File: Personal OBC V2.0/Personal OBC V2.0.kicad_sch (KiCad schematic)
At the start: 13 parts, among them J2 Screw_Terminal_01x06, U1 STM32F042G6Ux, U2 MS560702BA03-50, U3 AP2210N-3.3TRG1

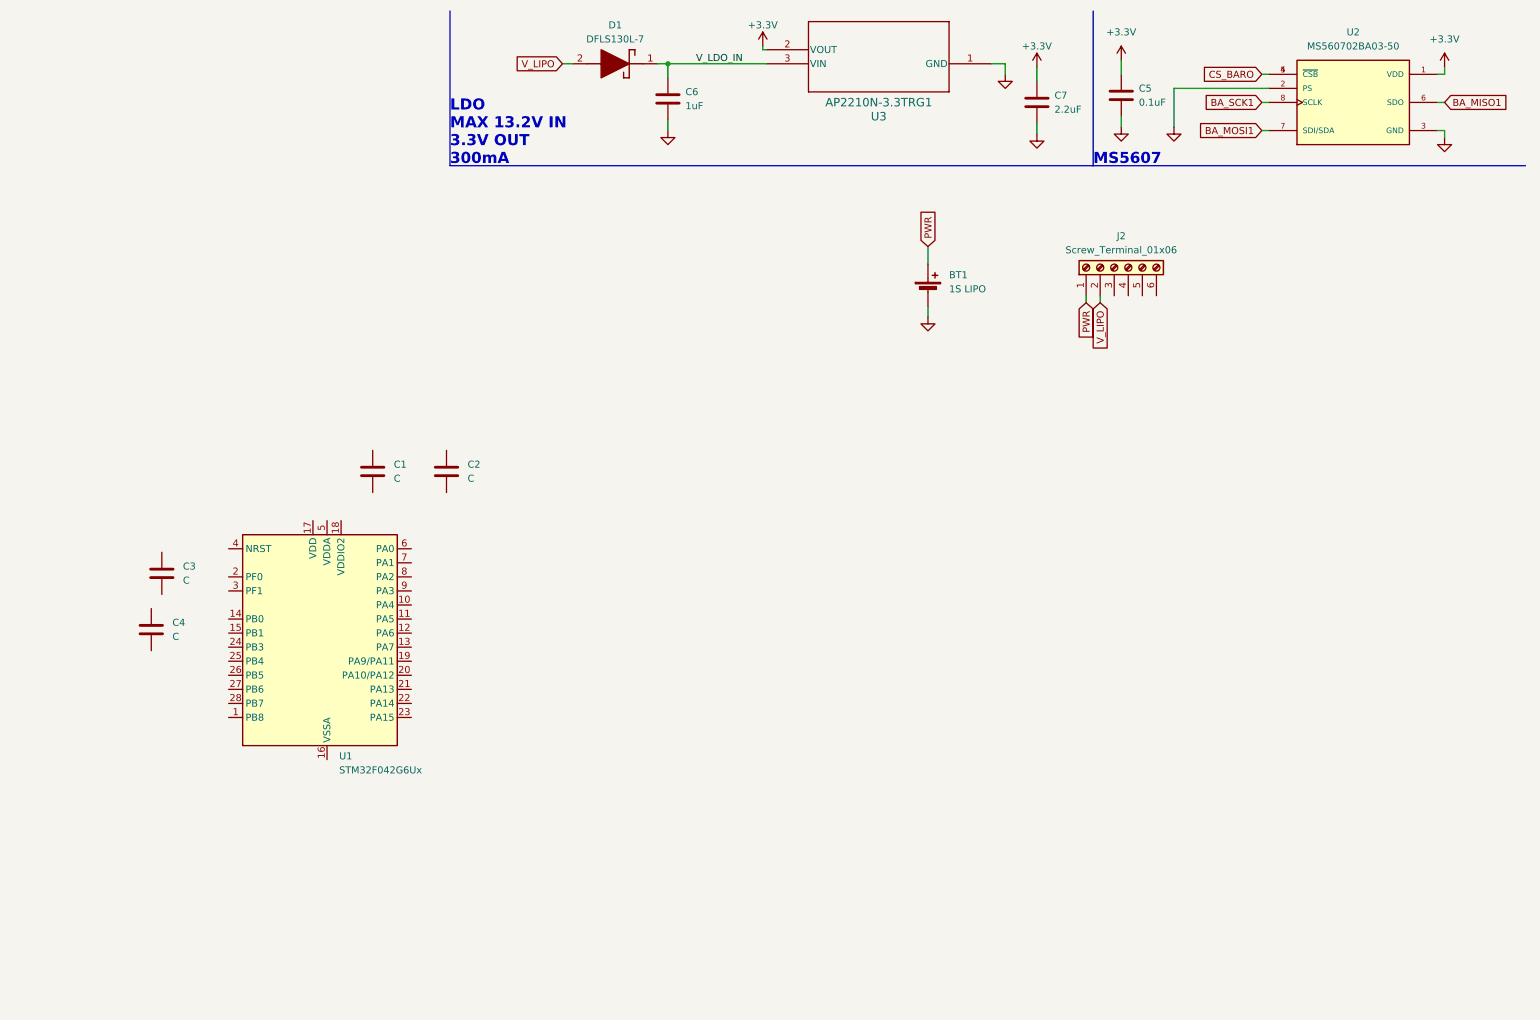
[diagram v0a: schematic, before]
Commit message: Aaaaaa
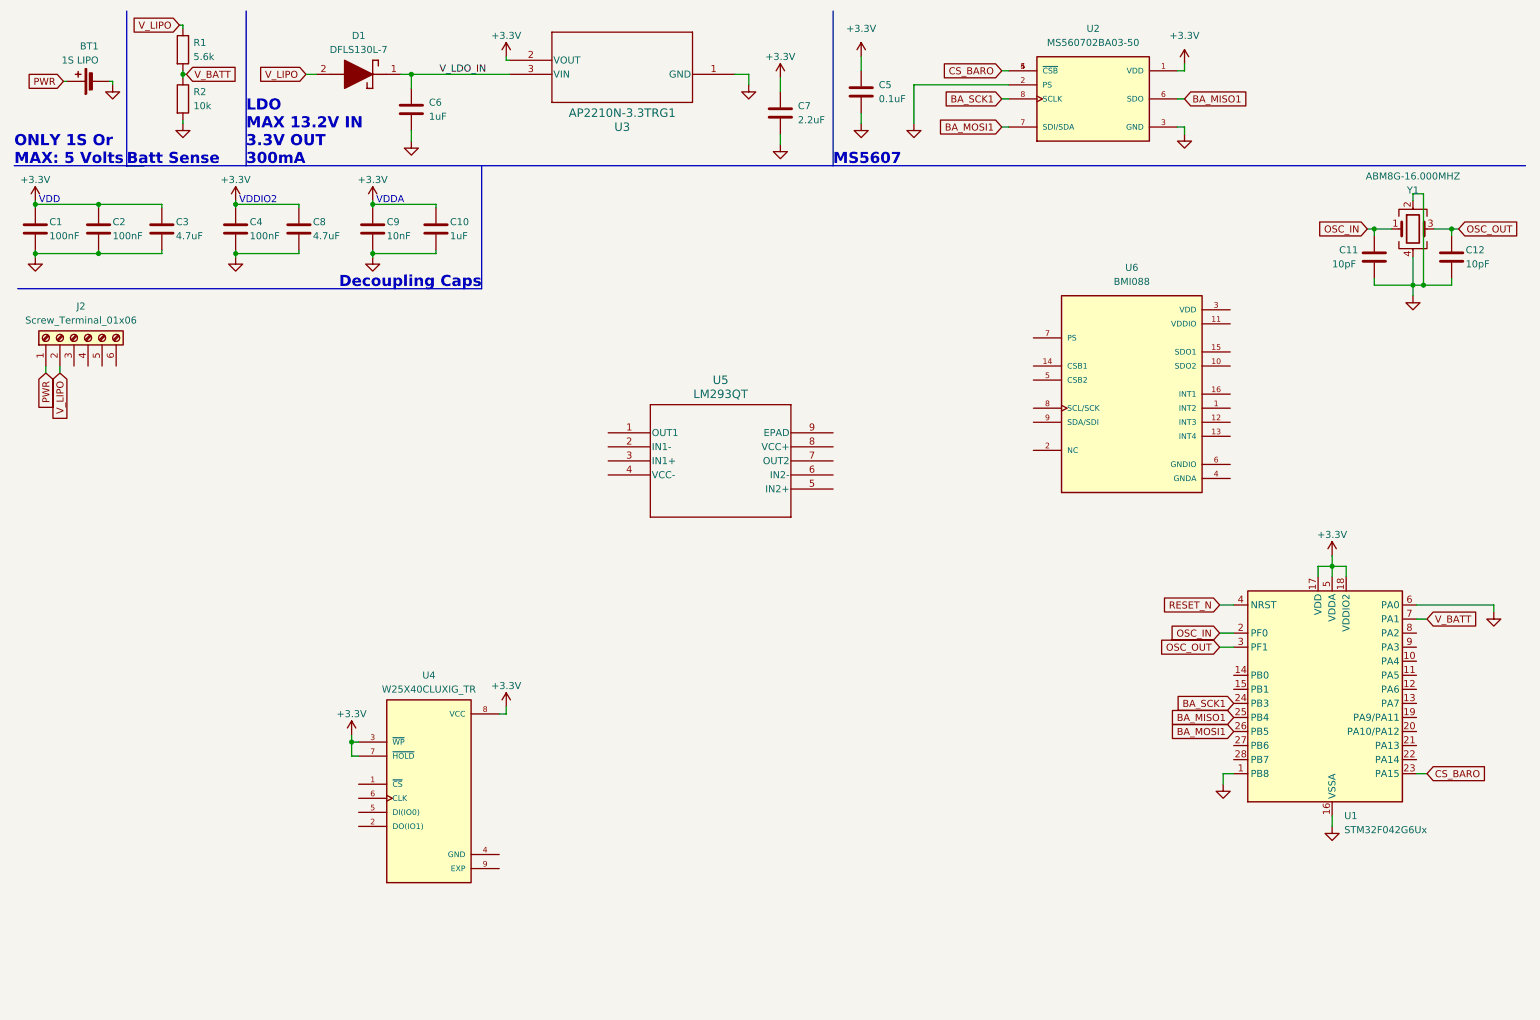
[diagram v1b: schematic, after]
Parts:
- added C10: 1uF, symbol Device:C
- added C11, C12: 10pF, symbol Device:C
- added C8: 4.7uF, symbol Device:C
- added C9: 10nF, symbol Device:C
- added R1: 5.6k, symbol Device:R
- added R2: 10k, symbol Device:R
- added U4: W25X40CLUXIG_TR, W25X40CLUXIG_TR:PSON50P300X200X60-9N, symbol W25X40CLUXIG TR:W25X40CLUXIG_TR
- added U5: LM293QT, DFN8_2P16X2P16X0P5_STM, symbol LM293QT:LM293QT
- added U6: BMI088, BMI088:PQFN50P450X300X100-16N, symbol BMI088:BMI088
- added Y1: ABM8G-16.000MHZ, Crystal:Crystal_SMD_Abracon_ABM8G-4Pin_3.2x2.5mm, symbol Device:Crystal_GND24
- C1, C2, C4: value C -> 100nF
- C3: value C -> 4.7uF
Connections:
- net +3.3V: now also C1.1, C2.1, C3.1, C4.1, U1.17 (VDD), U1.18 (VDDIO2), U1.5 (VDDA), C10.1, C8.1, C9.1, U4.3 (~{WP}), U4.7 (~{HOLD}), U4.8 (VCC)
- net BA_MISO1: now also U1.25 (PB4)
- net BA_MOSI1: now also U1.26 (PB5)
- net BA_SCK1: now also U1.24 (PB3)
- net CS_BARO: now also U1.23 (PA15)
- net GND: now also C1.2, C2.2, C3.2, C4.2, U1.1 (PB8), U1.16 (VSSA), U1.6 (PA0), C10.2, C11.2, C12.2, C8.2, C9.2, R2.2, Y1.2, Y1.4
- net V_LIPO: now also R1.1
- net OSC_IN: now reaches U1.2 (PF0)
- net OSC_IN: now also C11.1, Y1.1
- net OSC_OUT: now reaches U1.3 (PF1)
- net OSC_OUT: now also C12.1, Y1.3
- net RESET_N: now reaches U1.4 (NRST)
- net V_BATT: now reaches U1.7 (PA1)
- net V_BATT: now also R1.2, R2.1
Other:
- note added: "Batt Sense"
- note added: "Decoupling Caps"
- note added: "ONLY 1S Or MAX: 5 Volts"
- note added: "VDD"
- note added: "VDDA"
- note added: "VDDIO2"
- moved on the sheet: BT1, C1, C2, C3, C4, C5, C6, C7, D1, J2, U1, U2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

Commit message: Piss bot
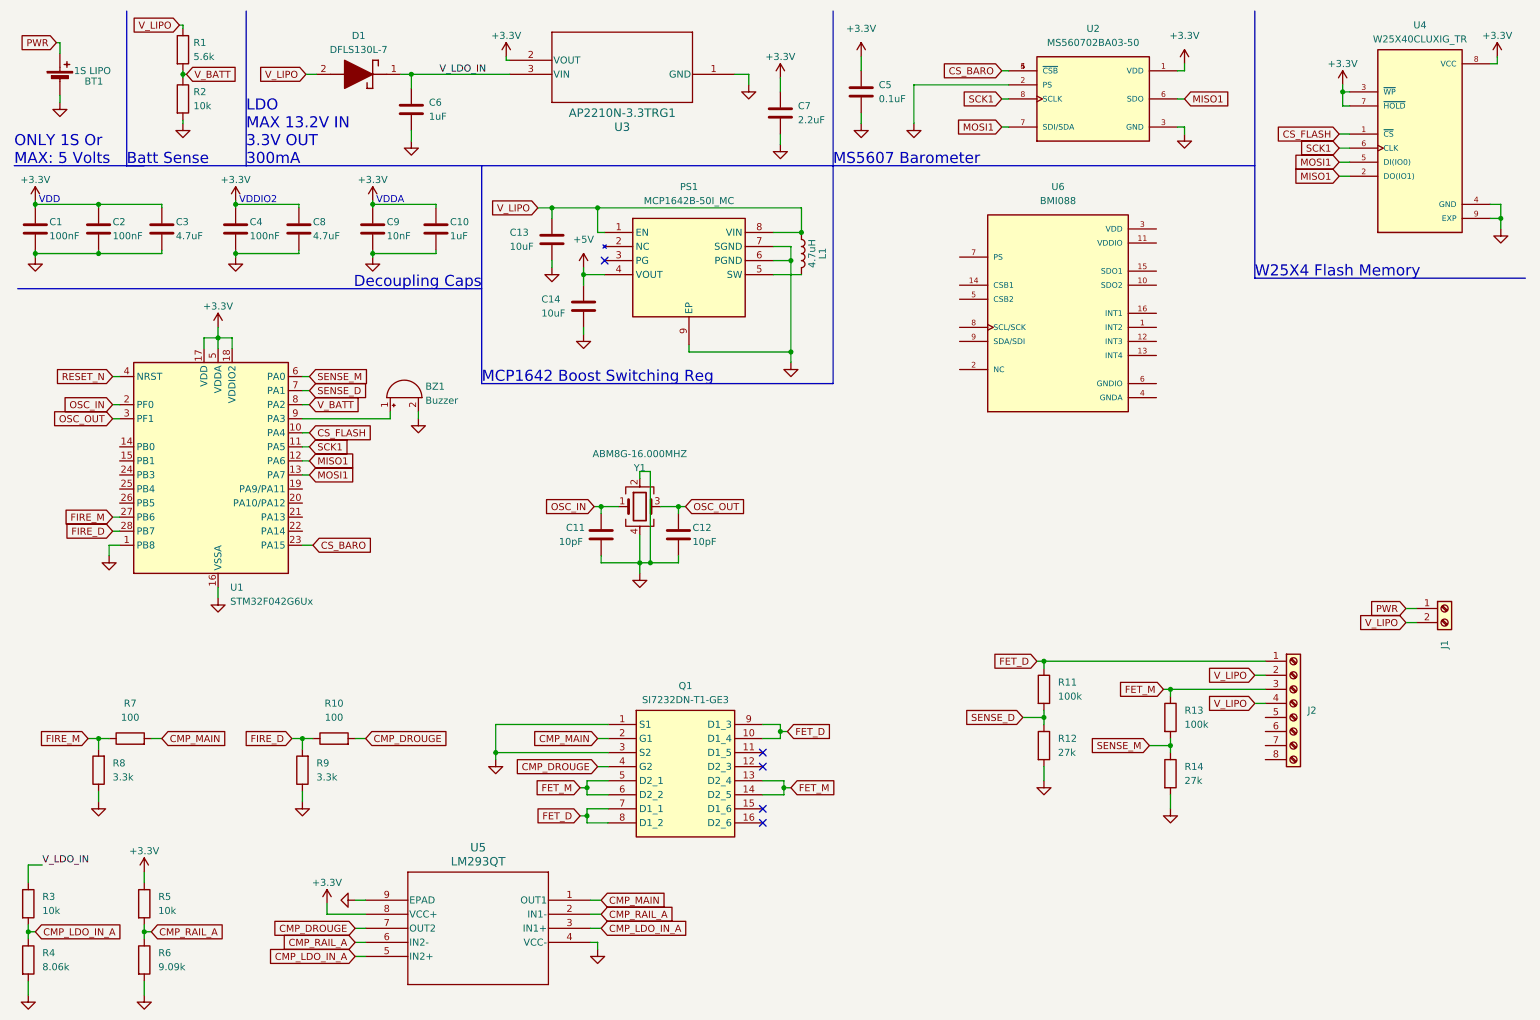
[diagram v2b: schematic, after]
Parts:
- removed J2: Screw_Terminal_01x06, symbol Connector:Screw_Terminal_01x06
- added BZ1: Buzzer, symbol Device:Buzzer
- added C13, C14: 10uF, symbol Device:C
- added J1: Screw_Terminal_01x02, symbol Connector:Screw_Terminal_01x02
- added J2: Screw_Terminal_01x04, symbol Connector:Screw_Terminal_01x08
- added L1: 4.7uH, symbol Device:L
- added PS1: MCP1642B-50I_MC, SON50P300X200X100-9N-D, symbol MCP1642B-50I_MC:MCP1642B-50I_MC
- added Q1: SI7232DN-T1-GE3, SI7232DNT1GE3, symbol SI7232DN-T1-GE3:SI7232DN-T1-GE3
- added R10, R7: 100, symbol Device:R
- added R11, R13: 100k, symbol Device:R
- added R12, R14: 27k, symbol Device:R
- added R3, R5: 10k, symbol Device:R
- added R4: 8.06k, symbol Device:R
- added R6: 9.09k, symbol Device:R
- added R8, R9: 3.3k, symbol Device:R
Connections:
- net +3.3V: now also U5.8 (VCC+), R5.1
- net GND: now also U4.4 (GND), U4.9 (EXP), U5.4 (VCC-), U5.9 (EPAD), BZ1.2 (+), C13.2, C14.2, PS1.6 (PGND), PS1.7 (SGND), PS1.9 (EP), Q1.1 (S1), Q1.3 (S2), R12.2, R14.2, R4.2, R6.2, R8.1, R9.1; no longer U1.6 (PA0)
- net PWR: now also J1.1 (Pin_1)
- net V_BATT: now also U1.8 (PA2); no longer U1.7 (PA1)
- net V_LDO_IN: now also R3.1
- net V_LIPO: now also C13.1, J1.2 (Pin_2), J2.2 (Pin_2), J2.4 (Pin_4), L1.1, PS1.1 (EN), PS1.8 (VIN)
- net CS_FLASH: now reaches U1.10 (PA4)
- net CS_FLASH: now also U4.1 (~{CS})
- net SCK1: now reaches U1.11 (PA5)
- net SCK1: now also U2.8 (SCLK), U4.6 (CLK)
- net MISO1: now reaches U1.12 (PA6)
- net MISO1: now also U2.6 (SDO), U4.2 (DO(IO1))
- net MOSI1: now reaches U1.13 (PA7)
- net MOSI1: now also U2.7 (SDI/SDA), U4.5 (DI(IO0))
- net FIRE_M: now reaches U1.27 (PB6)
- net FIRE_M: now also R7.1, R8.2
- net FIRE_D: now reaches U1.28 (PB7)
- net FIRE_D: now also R10.1, R9.2
- net at U1.9 (PA3): now also BZ1.1 (-)
- net CMP_MAIN: now reaches U5.1 (OUT1)
- net CMP_MAIN: now also Q1.2 (G1), R7.2
- net CMP_RAIL_A: now reaches U5.2 (IN1-)
- net CMP_RAIL_A: now also U5.6 (IN2-), R5.2, R6.1
- net CMP_LDO_IN_A: now reaches U5.3 (IN1+)
- net CMP_LDO_IN_A: now also U5.5 (IN2+), R3.2, R4.1
- net CMP_DROUGE: now reaches U5.7 (OUT2)
- net CMP_DROUGE: now also Q1.4 (G2), R10.2
- net BA_MISO1: no longer names the net of U1.25 (PB4)
- net BA_MISO1: no longer U2.6 (SDO)
- net BA_MOSI1: no longer names the net of U1.26 (PB5)
- net BA_MOSI1: no longer U2.7 (SDI/SDA)
- net BA_SCK1: no longer names the net of U1.24 (PB3)
- net BA_SCK1: no longer U2.8 (SCLK)
- new net: L1.2, PS1.5 (SW)
- new net +5V: C14.1, PS1.4 (VOUT)
- new net FET_D: J2.1 (Pin_1), Q1.10 (D1_4), Q1.7 (D1_1), Q1.8 (D1_2), Q1.9 (D1_3), R11.1
- new net FET_M: J2.3 (Pin_3), Q1.13 (D2_4), Q1.14 (D2_5), Q1.5 (D2_1), Q1.6 (D2_2), R13.1
- new net SENSE_D: R11.2, R12.1, U1.7 (PA1)
- new net SENSE_M: R13.2, R14.1, U1.6 (PA0)
- no-connect marks 0 -> 5
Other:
- note added: "MCP1642 Boost Switching Reg"
- note added: "MS5607 Barometer"
- note added: "W25X4 Flash Memory"
- note removed: "MS5607"
- moved on the sheet: BT1, C11, C12, U1, U4, U5, U6, Y1

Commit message: AAAA
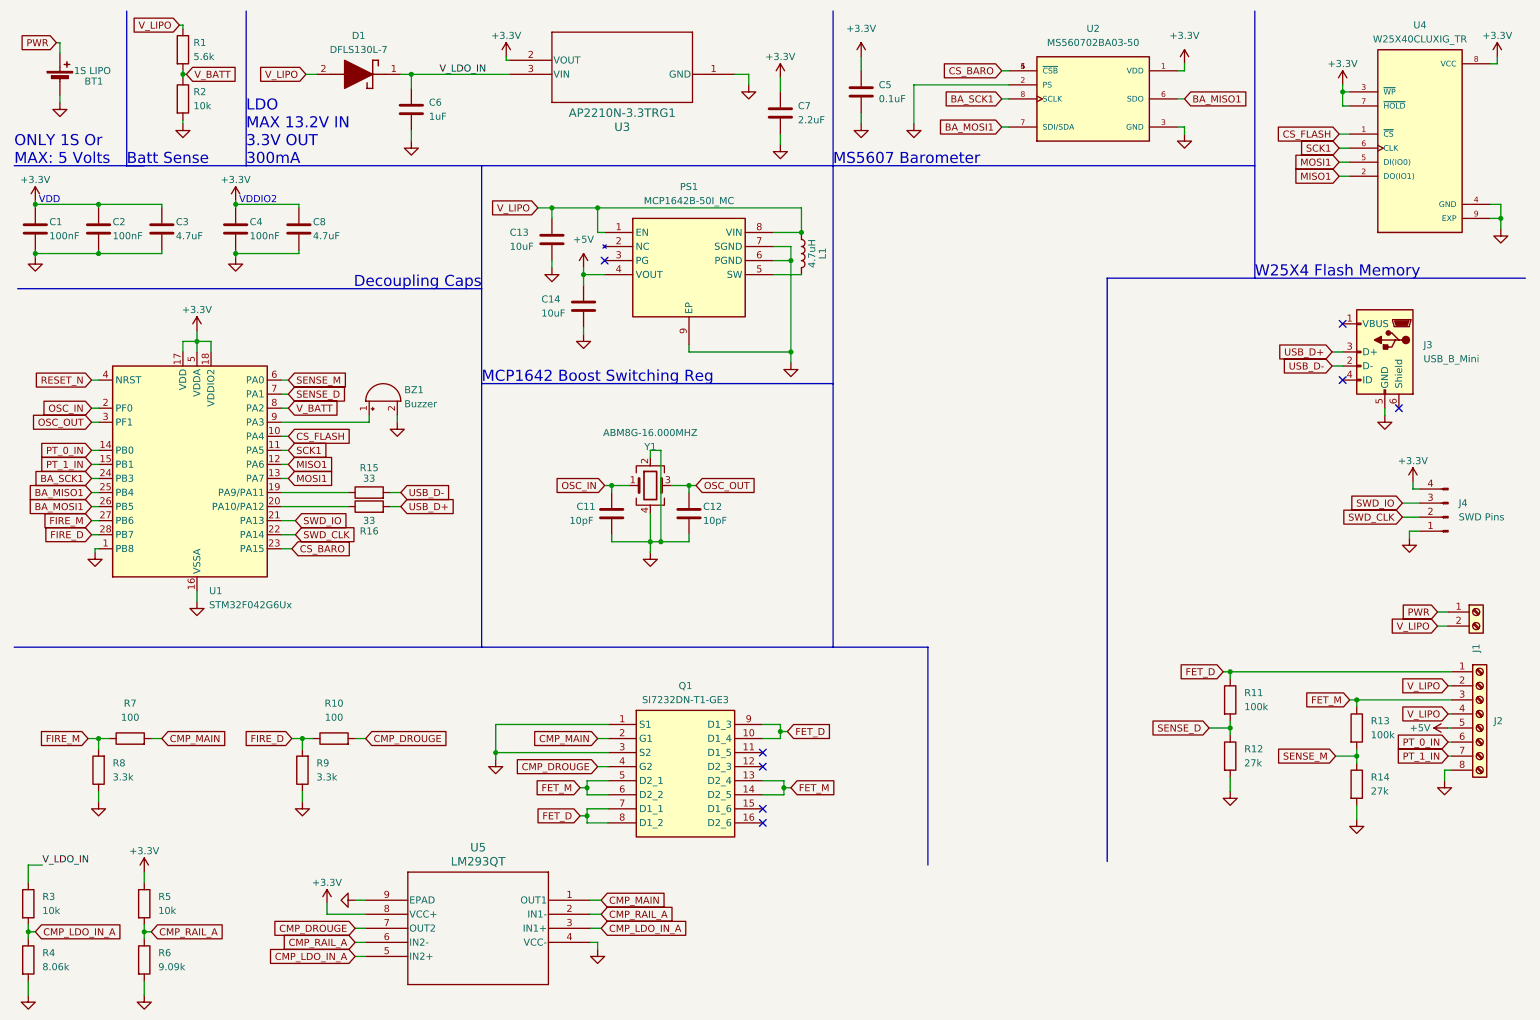
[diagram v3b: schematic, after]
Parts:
- removed C10: 1uF, symbol Device:C
- removed C9: 10nF, symbol Device:C
- removed U6: BMI088, BMI088:PQFN50P450X300X100-16N, symbol BMI088:BMI088
- added J3: USB_B_Mini, Connector_USB:USB_Micro-AB_Molex_47590-0001, symbol Connector:USB_B_Mini
- added J4: SWD Pins, symbol Connector:Conn_01x04_Pin
- added R15, R16: 33, symbol Device:R
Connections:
- net +3.3V: now also J4.4 (Pin_4)
- net +5V: now also J2.5 (Pin_5)
- net GND: now also J2.8 (Pin_8), J3.5 (GND), J4.1 (Pin_1)
- net MISO1: no longer U2.6 (SDO)
- net MOSI1: no longer U2.7 (SDI/SDA)
- net SCK1: no longer U2.8 (SCLK)
- net PT_0_IN: now reaches J2.6 (Pin_6)
- net PT_0_IN: now also U1.14 (PB0)
- net PT_1_IN: now reaches J2.7 (Pin_7)
- net PT_1_IN: now also U1.15 (PB1)
- net at U1.19 (PA9/PA11): now also R15.1
- net at U1.20 (PA10/PA12): now also R16.1
- net SWD_IO: now reaches U1.21 (PA13)
- net SWD_IO: now also J4.3 (Pin_3)
- net SWD_CLK: now reaches U1.22 (PA14)
- net SWD_CLK: now also J4.2 (Pin_2)
- net BA_SCK1: now reaches U1.24 (PB3)
- net BA_SCK1: now also U2.8 (SCLK)
- net BA_MISO1: now reaches U1.25 (PB4)
- net BA_MISO1: now also U2.6 (SDO)
- net BA_MOSI1: now reaches U1.26 (PB5)
- net BA_MOSI1: now also U2.7 (SDI/SDA)
- new net USB_D+: J3.3 (D+), R16.2
- new net USB_D-: J3.2 (D-), R15.2
- no-connect marks 5 -> 8
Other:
- note removed: "VDDA"
- moved on the sheet: BZ1, C11, C12, J1, J2, R11, R12, R13, R14, U1, Y1

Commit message: Aaaaaa
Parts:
- BT1: footprint (none) -> Connector_JST:JST_PH_S2B-PH-K_1x02_P2.00mm_Horizontal
- BZ1: footprint (none) -> Buzzer_Beeper:Buzzer_TDK_PS1240P02BT_D12.2mm_H6.5mm
- C1, C11, C12, C2, C3, C4, C5, C6, C7, C8: footprint (none) -> Capacitor_SMD:C_0402_1005Metric
- C13, C14: footprint (none) -> Capacitor_SMD:C_0603_1608Metric
- D1: footprint DFLS130L7 -> DFLS130L-7:DFLS130L7
- J1: footprint (none) -> TerminalBlock_TE-Connectivity:TerminalBlock_TE_282834-2_1x02_P2.54mm_Horizontal
- J2: footprint (none) -> TerminalBlock_TE-Connectivity:TerminalBlock_TE_282834-8_1x08_P2.54mm_Horizontal
- J4: footprint (none) -> Connector_PinHeader_2.54mm:PinHeader_1x04_P2.54mm_Vertical
- L1: footprint (none) -> Inductor_SMD:L_1008_2520Metric
- PS1: footprint SON50P300X200X100-9N-D -> MCP1642B-50I_MC:SON50P300X200X100-9N-D
- Q1: footprint SI7232DNT1GE3 -> SI7232DN-T1-GE3:SI7232DNT1GE3
- R1, R10, R11, R12, R13, R14, R15, R16, R2, R3, R4, R5, R6, R7, R8, R9: footprint (none) -> Resistor_SMD:R_0402_1005Metric
- U3: footprint SOT_3.3TRG1_DIO -> AP2210N_3_3TRG1:SOT_3.3TRG1_DIO
- U5: footprint DFN8_2P16X2P16X0P5_STM -> LM293QT:DFN8_2P16X2P16X0P5_STM
